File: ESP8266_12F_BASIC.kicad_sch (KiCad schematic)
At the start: 35 parts, among them J1 Conn_01x02_Male, J2 Conn_01x04_Male, Q1 BC547, U1 ESP-12F, U2 AP1117-33

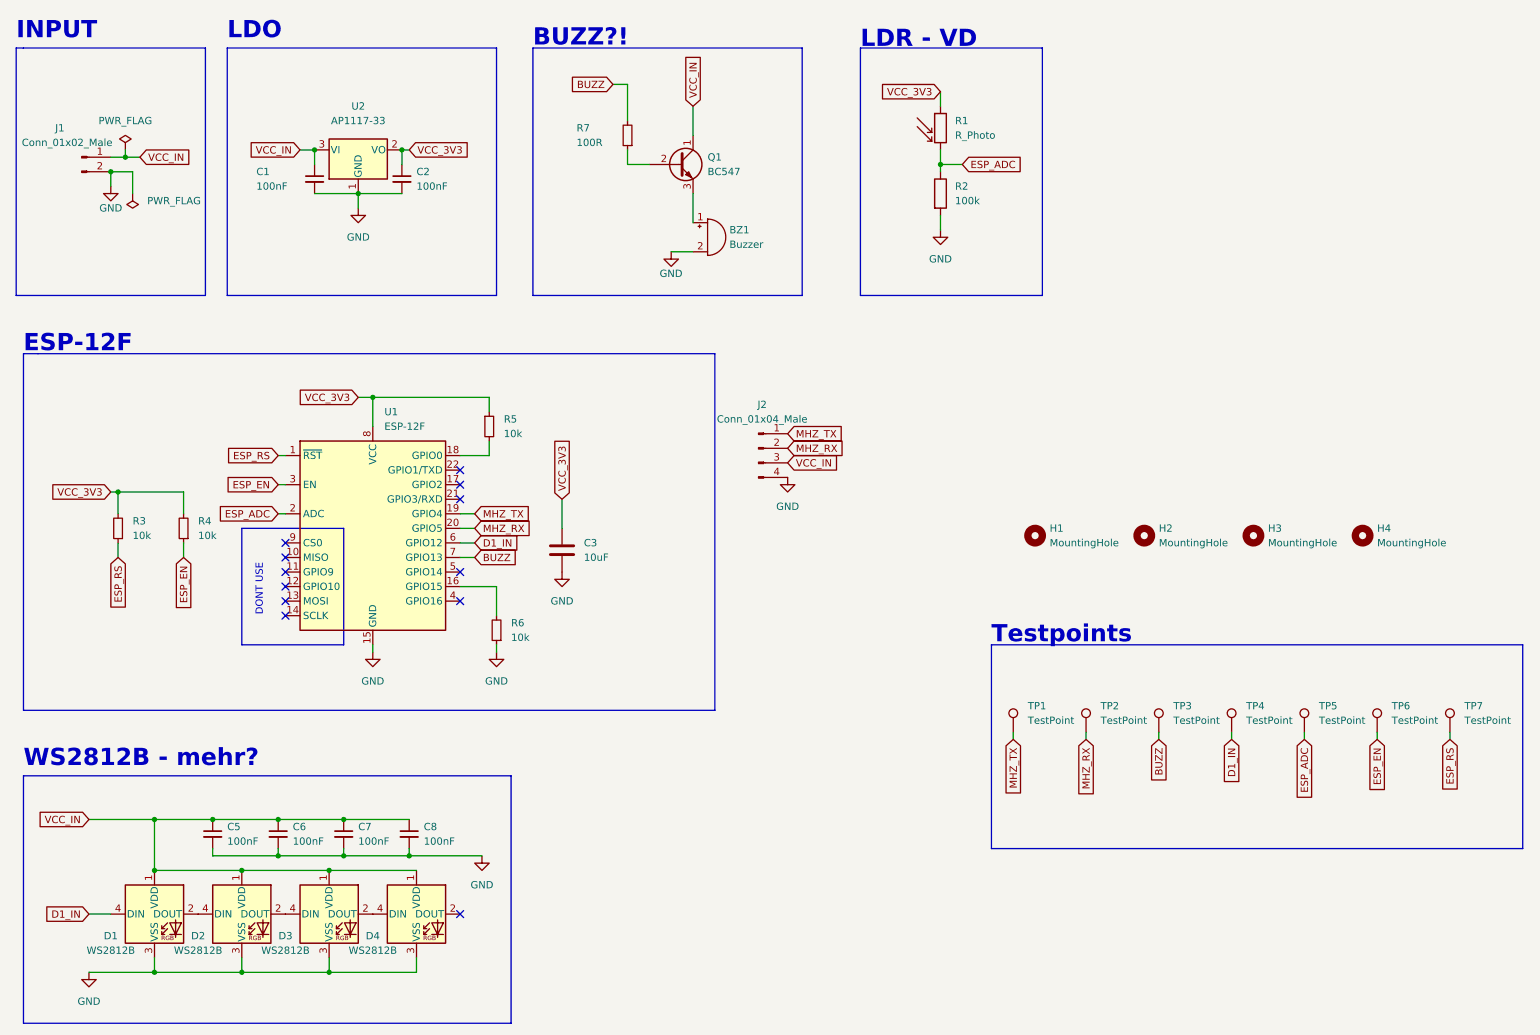
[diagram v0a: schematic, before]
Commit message: major fixes
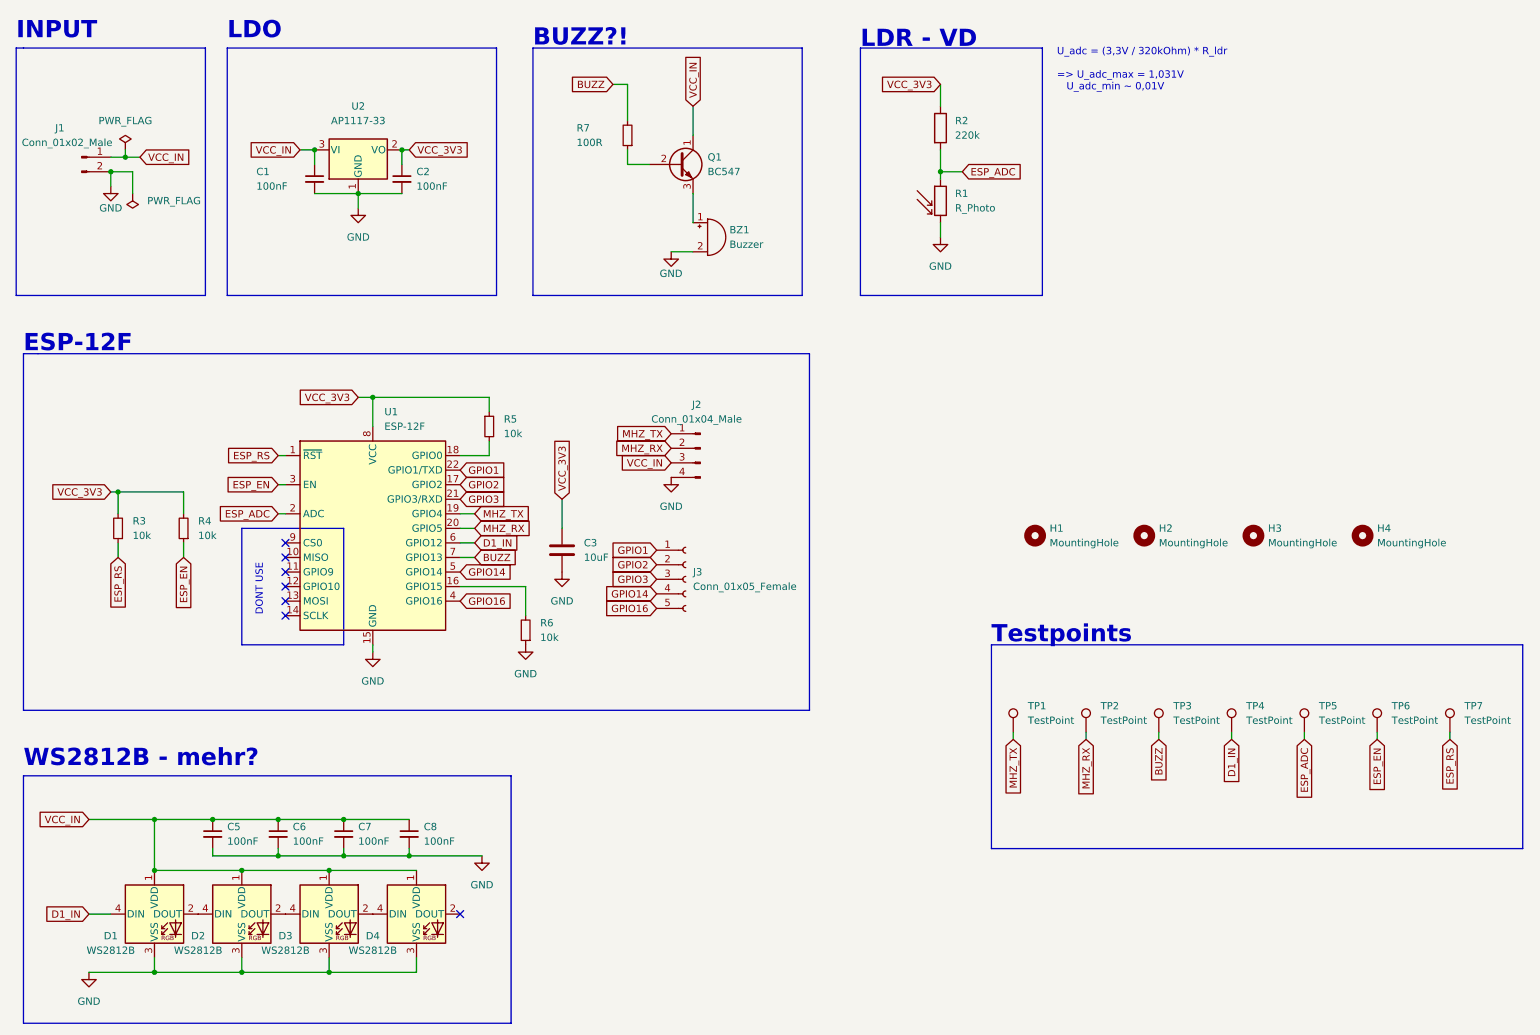
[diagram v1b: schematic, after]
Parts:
- added J3: Conn_01x05_Female, Connector_PinHeader_2.54mm:PinHeader_1x05_P2.54mm_Vertical, symbol Connector:Conn_01x05_Female
- R2: value 100k -> 220k
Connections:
- net ESP_ADC: now also R1.1, R2.2; no longer R1.2, R2.1
- net GND: now also R1.2; no longer R2.2
- net VCC_3V3: now also R2.1; no longer R1.1
- net GPIO2: now reaches U1.17 (GPIO2)
- net GPIO2: now also J3.2 (Pin_2)
- net GPIO3: now reaches U1.21 (GPIO3/RXD)
- net GPIO3: now also J3.3 (Pin_3)
- net GPIO1: now reaches U1.22 (GPIO1/TXD)
- net GPIO1: now also J3.1 (Pin_1)
- net GPIO16: now reaches U1.4 (GPIO16)
- net GPIO16: now also J3.5 (Pin_5)
- net GPIO14: now reaches U1.5 (GPIO14)
- net GPIO14: now also J3.4 (Pin_4)
- no-connect marks 12 -> 7
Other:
- note added: "U_adc = (3,3V / 320kOhm) * R_ldr => U_adc_max = 1,031V U_adc_min ~ 0,01V"
- moved on the sheet: J2, R1, R6

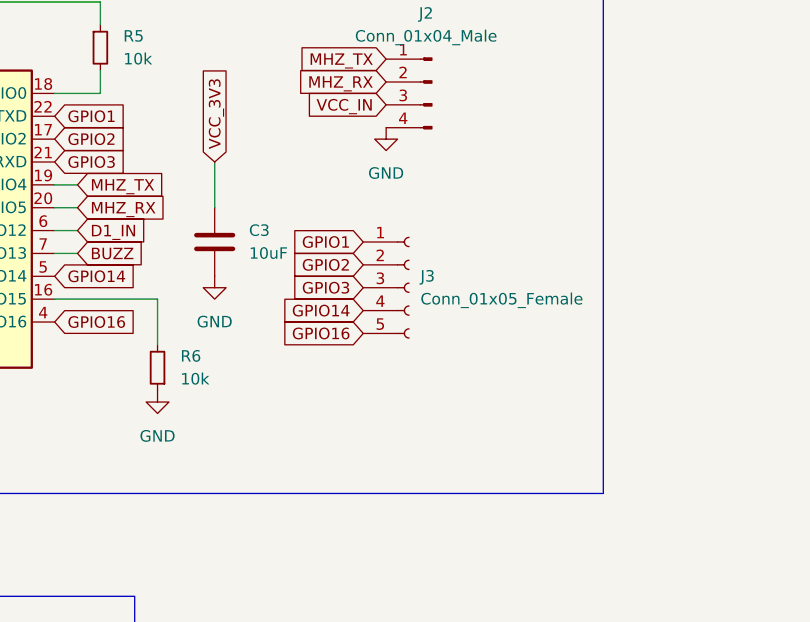
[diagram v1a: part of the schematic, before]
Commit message: caps added and move also added new picture
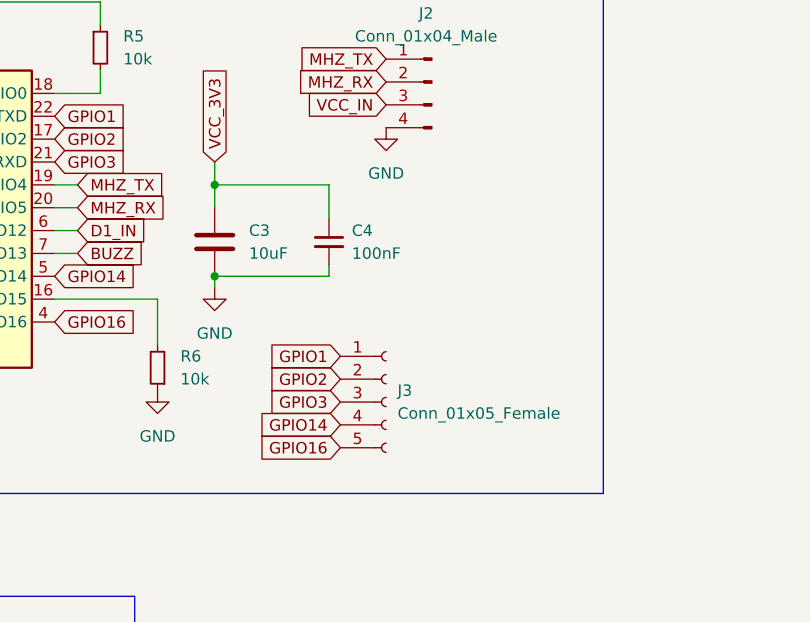
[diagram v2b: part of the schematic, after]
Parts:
- added C4: 100nF, Capacitor_SMD:C_1206_3216Metric_Pad1.33x1.80mm_HandSolder, symbol Device:C_Small
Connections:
- net GND: now also C4.2
- net VCC_3V3: now also C4.1
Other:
- moved on the sheet: J3
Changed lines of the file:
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@@
   (junction (at 76.2 48.26) (diameter 0) (color 0 0 0 0)
   )
+  (junction (at 111.76 114.3) (diameter 0) (color 0 0 0 0)
+  )
   (junction (at 73.66 163.83) (diameter 0) (color 0 0 0 0)
   )
   (junction (at 55.88 166.37) (diameter 0) (color 0 0 0 0)
+  )
+  (junction (at 111.76 104.14) (diameter 0) (color 0 0 0 0)
   )
   (junction (at 33.02 44.45) (diameter 0) (color 0 0 0 0)
@@
     (stroke (width 0) (type default) (color 0 0 0 0))
   )
+  (wire (pts (xy 124.46 113.03) (xy 124.46 114.3))
+    (stroke (width 0) (type default) (color 0 0 0 0))
+  )
   (wire (pts (xy 177.8 44.45) (xy 181.61 44.45))
     (stroke (width 0) (type default) (color 0 0 0 0))
@@
     (stroke (width 0) (type default) (color 0 0 0 0))
   )
+  (wire (pts (xy 111.76 115.57) (xy 111.76 114.3))
+    (stroke (width 0) (type default) (color 0 0 0 0))
+  )
   (wire (pts (xy 99.06 83.82) (xy 78.74 83.82))
     (stroke (width 0) (type default) (color 0 0 0 0))
@@
     (stroke (width 0) (type default) (color 0 0 0 0))
   )
-  (wire (pts (xy 111.76 101.6) (xy 111.76 106.68))
+  (wire (pts (xy 111.76 101.6) (xy 111.76 104.14))
+    (stroke (width 0) (type default) (color 0 0 0 0))
+  )
+  (wire (pts (xy 124.46 107.95) (xy 124.46 104.14))
     (stroke (width 0) (type default) (color 0 0 0 0))
   )
@@
     (stroke (width 0) (type default) (color 0 0 0 0))
   )
+  (wire (pts (xy 111.76 104.14) (xy 111.76 106.68))
+    (stroke (width 0) (type default) (color 0 0 0 0))
+  )
   (polyline (pts (xy 154.94 138.43) (xy 17.78 138.43))
     (stroke (width 0) (type default) (color 0 0 0 0))
@@
     (stroke (width 0) (type default) (color 0 0 0 0))
   )
+  (wire (pts (xy 124.46 104.14) (xy 111.76 104.14))
+    (stroke (width 0) (type default) (color 0 0 0 0))
+  )
   (wire (pts (xy 93.98 111.76) (xy 96.52 111.76))
     (stroke (width 0) (type default) (color 0 0 0 0))
@@
   )
   (polyline (pts (xy 163.83 22.86) (xy 163.83 66.04))
+    (stroke (width 0) (type default) (color 0 0 0 0))
+  )
+  (wire (pts (xy 111.76 114.3) (xy 124.46 114.3))
     (stroke (width 0) (type default) (color 0 0 0 0))
   )
@@
     )
   )
-  (global_label "GPIO2" (shape input) (at 128.27 113.03 180) (fields_autoplaced)
-    (effects (font (size 1.27 1.27)) (justify right))
-    (property "Intersheet References" "${INTERSHEET_REFS}" (id 0) (at 120.1721 113.1094 0)
+  (global_label "GPIO2" (shape input) (at 125.73 125.73 180) (fields_autoplaced)
+    (effects (font (size 1.27 1.27)) (justify right))
+    (property "Intersheet References" "${INTERSHEET_REFS}" (id 0) (at 117.6321 125.8094 0)
       (effects (font (size 1.27 1.27)) (justify right) hide)
     )
@@
     )
   )
-  (global_label "GPIO1" (shape input) (at 128.27 110.49 180) (fields_autoplaced)
-    (effects (font (size 1.27 1.27)) (justify right))
-    (property "Intersheet References" "${INTERSHEET_REFS}" (id 0) (at 120.1721 110.5694 0)
-      (effects (font (size 1.27 1.27)) (justify right) hide)
-    )
-  )
-  (global_label "GPIO14" (shape input) (at 128.27 118.11 180) (fields_autoplaced)
-    (effects (font (size 1.27 1.27)) (justify right))
-    (property "Intersheet References" "${INTERSHEET_REFS}" (id 0) (at 118.9626 118.1894 0)
+  (global_label "GPIO1" (shape input) (at 125.73 123.19 180) (fields_autoplaced)
+    (effects (font (size 1.27 1.27)) (justify right))
+    (property "Intersheet References" "${INTERSHEET_REFS}" (id 0) (at 117.6321 123.2694 0)
+      (effects (font (size 1.27 1.27)) (justify right) hide)
+    )
+  )
+  (global_label "GPIO14" (shape input) (at 125.73 130.81 180) (fields_autoplaced)
+    (effects (font (size 1.27 1.27)) (justify right))
+    (property "Intersheet References" "${INTERSHEET_REFS}" (id 0) (at 116.4226 130.8894 0)
       (effects (font (size 1.27 1.27)) (justify right) hide)
     )
@@
     )
   )
-  (global_label "GPIO3" (shape input) (at 128.27 115.57 180) (fields_autoplaced)
-    (effects (font (size 1.27 1.27)) (justify right))
-    (property "Intersheet References" "${INTERSHEET_REFS}" (id 0) (at 120.1721 115.6494 0)
+  (global_label "GPIO3" (shape input) (at 125.73 128.27 180) (fields_autoplaced)
+    (effects (font (size 1.27 1.27)) (justify right))
+    (property "Intersheet References" "${INTERSHEET_REFS}" (id 0) (at 117.6321 128.3494 0)
       (effects (font (size 1.27 1.27)) (justify right) hide)
     )
@@
     )
   )
-  (global_label "GPIO16" (shape input) (at 128.27 120.65 180) (fields_autoplaced)
-    (effects (font (size 1.27 1.27)) (justify right))
-    (property "Intersheet References" "${INTERSHEET_REFS}" (id 0) (at 118.9626 120.7294 0)
+  (global_label "GPIO16" (shape input) (at 125.73 133.35 180) (fields_autoplaced)
+    (effects (font (size 1.27 1.27)) (justify right))
+    (property "Intersheet References" "${INTERSHEET_REFS}" (id 0) (at 116.4226 133.4294 0)
       (effects (font (size 1.27 1.27)) (justify right) hide)
     )
@@
     (pin "2")
   )
-  (symbol (lib_id "Connector:Conn_01x05_Female") (at 133.35 115.57 0) (unit 1)
-    (in_bom yes) (on_board yes) (fields_autoplaced)
-    (property "Reference" "J3" (id 0) (at 134.62 114.2999 0)
-      (effects (font (size 1.27 1.27)) (justify left))
-    )
-    (property "Value" "Conn_01x05_Female" (id 1) (at 134.62 116.8399 0)
-      (effects (font (size 1.27 1.27)) (justify left))
-    )
-    (property "Footprint" "Connector_PinHeader_2.54mm:PinHeader_1x05_P2.54mm_Vertical" (id 2) (at 133.35 115.57 0)
-      (effects (font (size 1.27 1.27)) hide)
-    )
-    (property "Datasheet" "~" (id 3) (at 133.35 115.57 0)
+  (symbol (lib_id "Connector:Conn_01x05_Female") (at 130.81 128.27 0) (unit 1)
+    (in_bom yes) (on_board yes) (fields_autoplaced)
+    (property "Reference" "J3" (id 0) (at 132.08 126.9999 0)
+      (effects (font (size 1.27 1.27)) (justify left))
+    )
+    (property "Value" "Conn_01x05_Female" (id 1) (at 132.08 129.5399 0)
+      (effects (font (size 1.27 1.27)) (justify left))
+    )
+    (property "Footprint" "Connector_PinHeader_2.54mm:PinHeader_1x05_P2.54mm_Vertical" (id 2) (at 130.81 128.27 0)
+      (effects (font (size 1.27 1.27)) hide)
+    )
+    (property "Datasheet" "~" (id 3) (at 130.81 128.27 0)
       (effects (font (size 1.27 1.27)) hide)
     )
@@
     (pin "4")
   )
+  (symbol (lib_id "Device:C_Small") (at 124.46 110.49 0) (unit 1)
+    (in_bom yes) (on_board yes) (fields_autoplaced)
+    (property "Reference" "C4" (id 0) (at 127 109.2262 0)
+      (effects (font (size 1.27 1.27)) (justify left))
+    )
+    (property "Value" "100nF" (id 1) (at 127 111.7662 0)
+      (effects (font (size 1.27 1.27)) (justify left))
+    )
+    (property "Footprint" "Capacitor_SMD:C_1206_3216Metric_Pad1.33x1.80mm_HandSolder" (id 2) (at 124.46 110.49 0)
+      (effects (font (size 1.27 1.27)) hide)
+    )
+    (property "Datasheet" "~" (id 3) (at 124.46 110.49 0)
+      (effects (font (size 1.27 1.27)) hide)
+    )
+    (pin "1")
+    (pin "2")
+  )
   (symbol (lib_id "Device:R_Small") (at 123.19 38.1 180) (unit 1)
     (in_bom yes) (on_board yes)
@@
     (pin "2")
   )
-  (symbol (lib_id "power:GND") (at 111.76 114.3 0) (unit 1)
-    (in_bom yes) (on_board yes) (fields_autoplaced)
-    (property "Reference" "#PWR06" (id 0) (at 111.76 120.65 0)
-      (effects (font (size 1.27 1.27)) hide)
-    )
-    (property "Value" "GND" (id 1) (at 111.76 119.38 0))
-    (property "Footprint" "" (id 2) (at 111.76 114.3 0)
-      (effects (font (size 1.27 1.27)) hide)
-    )
-    (property "Datasheet" "" (id 3) (at 111.76 114.3 0)
+  (symbol (lib_id "power:GND") (at 111.76 115.57 0) (unit 1)
+    (in_bom yes) (on_board yes) (fields_autoplaced)
+    (property "Reference" "#PWR06" (id 0) (at 111.76 121.92 0)
+      (effects (font (size 1.27 1.27)) hide)
+    )
+    (property "Value" "GND" (id 1) (at 111.76 120.65 0))
+    (property "Footprint" "" (id 2) (at 111.76 115.57 0)
+      (effects (font (size 1.27 1.27)) hide)
+    )
+    (property "Datasheet" "" (id 3) (at 111.76 115.57 0)
       (effects (font (size 1.27 1.27)) hide)
     )
@@
       (reference "C3") (unit 1) (value "10uF") (footprint "Capacitor_THT:CP_Radial_D6.3mm_P2.50mm")
     )
+    (path "/98303ac1-b7d5-40e4-aac5-5ff68116461f"
+      (reference "C4") (unit 1) (value "100nF") (footprint "Capacitor_SMD:C_1206_3216Metric_Pad1.33x1.80mm_HandSolder")
+    )
     (path "/9fbcf246-9897-43b2-ba86-188b08b53625"
